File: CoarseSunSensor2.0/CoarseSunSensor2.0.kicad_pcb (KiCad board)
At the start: 2 copper layers, 45.4 x 14.3 mm, 23 parts, among them IC1 ADS1115IDGSR, J1 53261-0571

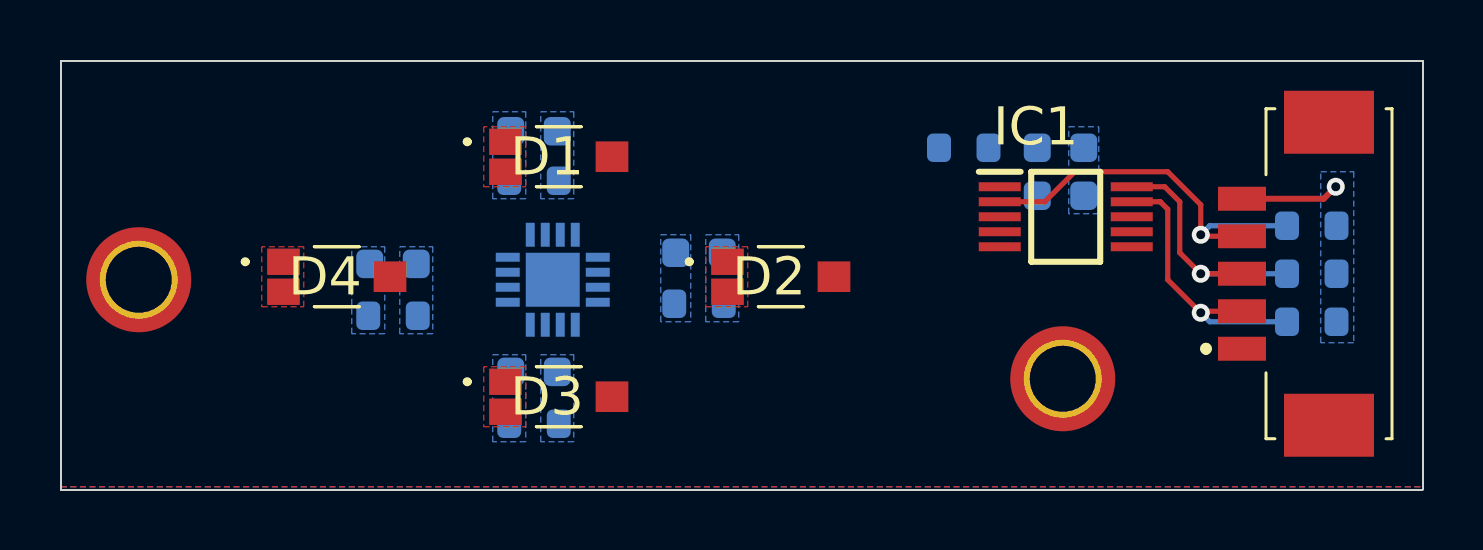
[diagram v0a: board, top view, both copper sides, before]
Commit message: Layout done
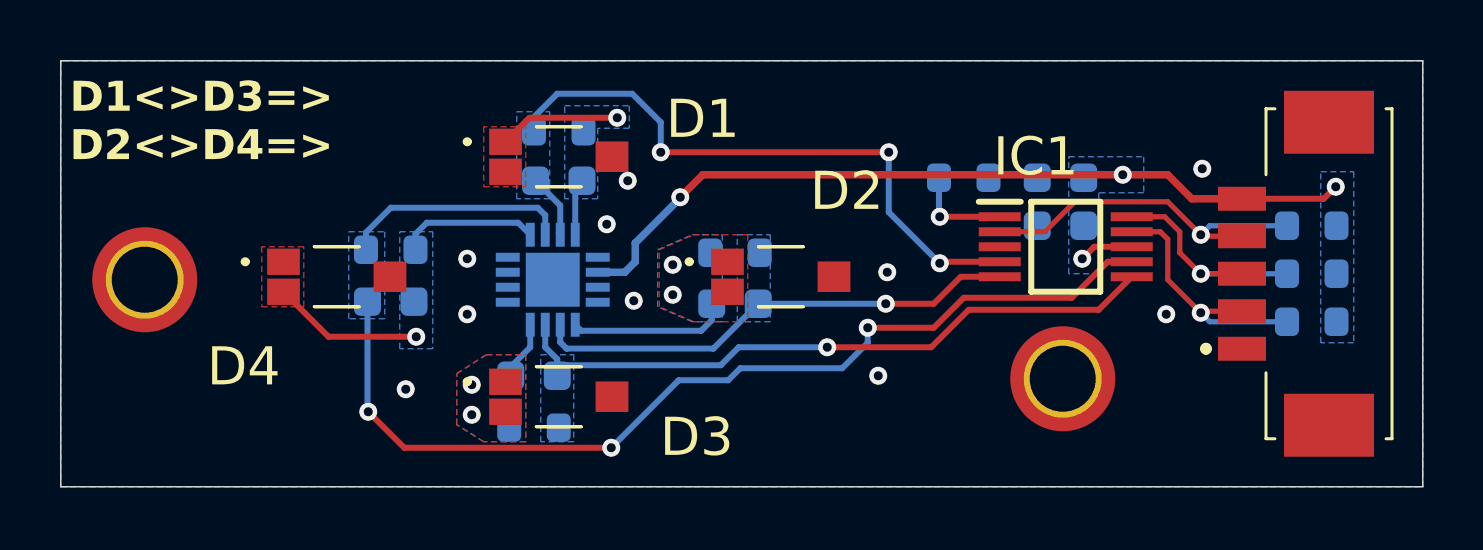
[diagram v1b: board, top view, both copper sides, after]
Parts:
- moved R4 2.20 mm to (147.8, 66.3), turned to 180 degrees
- moved C2 2.08 mm to (159.3, 68.1), turned to 0 degrees
- moved R2 2.08 mm to (159.3, 66.4), turned to 0 degrees
- moved C1 1.84 mm to (153.4, 64.0), turned to 180 degrees
- moved R1 1.84 mm to (153.4, 62.4), turned to 180 degrees
- moved C4 1.26 mm to (147.8, 68.0), turned to 180 degrees
- moved C5 1.00 mm to (170.1, 63.9)
- moved C6 1.00 mm to (170.1, 65.5)
- moved IC1 1.00 mm to (170.3, 66.2)
- moved R5 1.00 mm to (166.9, 63.9)
- moved H1 0.20 mm to (139.6, 67.3)
- moved R3 0.13 mm to (152.6, 72.2)
- moved C3 0.13 mm to (152.6, 70.5)
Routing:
- net /16bit I2C ADC/IN3: track 0.00 -> 40.1 mm, vias 0 -> 3
- net +3V3: track 3.29 -> 28.6 mm, vias 1 -> 4
- net /16bit I2C ADC/IN0: track 0.00 -> 22.7 mm, vias 0 -> 3
- net /16bit I2C ADC/IN2: track 0.00 -> 22.3 mm, vias 0 -> 1
- net /16bit I2C ADC/IN1: track 0.00 -> 16.3 mm, vias 0 -> 1
- net Net-(D4-ANODE_1): track 0.00 -> 9.72 mm, vias 0 -> 1
- net Net-(D1-ANODE_1): track 0.00 -> 5.95 mm, vias 0 -> 1
- net Net-(D2-ANODE_1): track 0.00 -> 5.33 mm, vias 0 -> 2
- net Net-(IC1-ADDR): track 0.00 -> 3.31 mm, vias 0 -> 1
- net Net-(D3-ANODE_1): track 0.00 -> 1.84 mm, vias 0 -> 2
- net /16bit I2C ADC/SDA: track 9.60 -> 8.60 mm
- net /16bit I2C ADC/alert/ready: track 13.0 -> 12.0 mm
- net /16bit I2C ADC/SLC: track 8.75 -> 7.75 mm
- net GND: vias 0 -> 10
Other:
- board size 45.4 x 14.3 mm -> 45.4 x 14.2 mm
- board text added: "D1<>D3=> D2<>D4=>"
- board text added: "Rev 1.0"
